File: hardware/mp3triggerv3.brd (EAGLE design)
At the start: 73.7 x 64.8 mm, 93 parts, among them J1 5.5x2.1mm Barrel, J10 M08X2, J3 USD-SOCKETNEW, J9 M10X2, U1 NCP1117, U2 MIC5323-3.3, U4 STM32F405RG, U5 PCM5100, U6 LM4990, Y1 8MHz

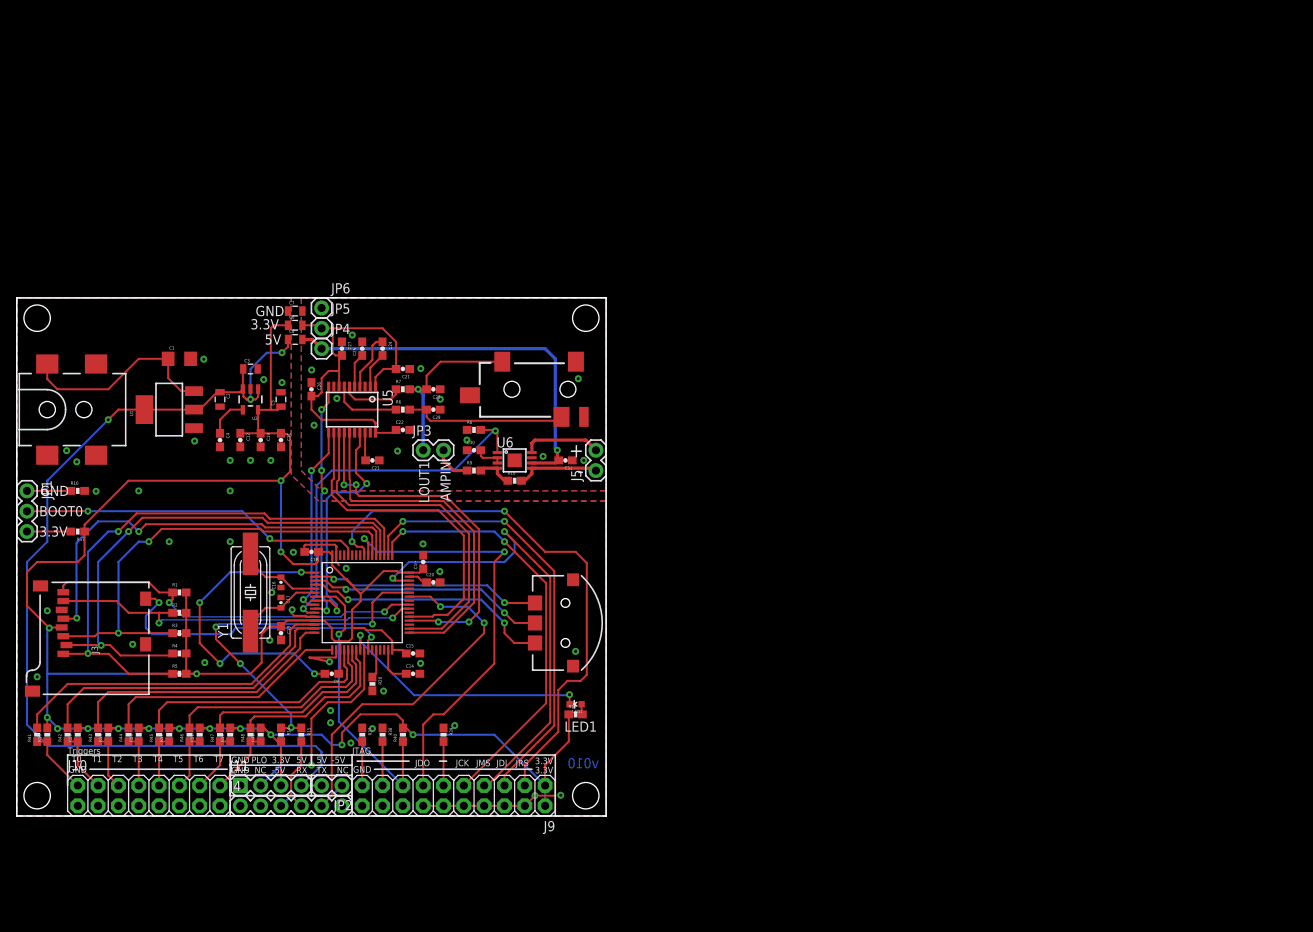
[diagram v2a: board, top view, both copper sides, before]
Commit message: v31, ready for review
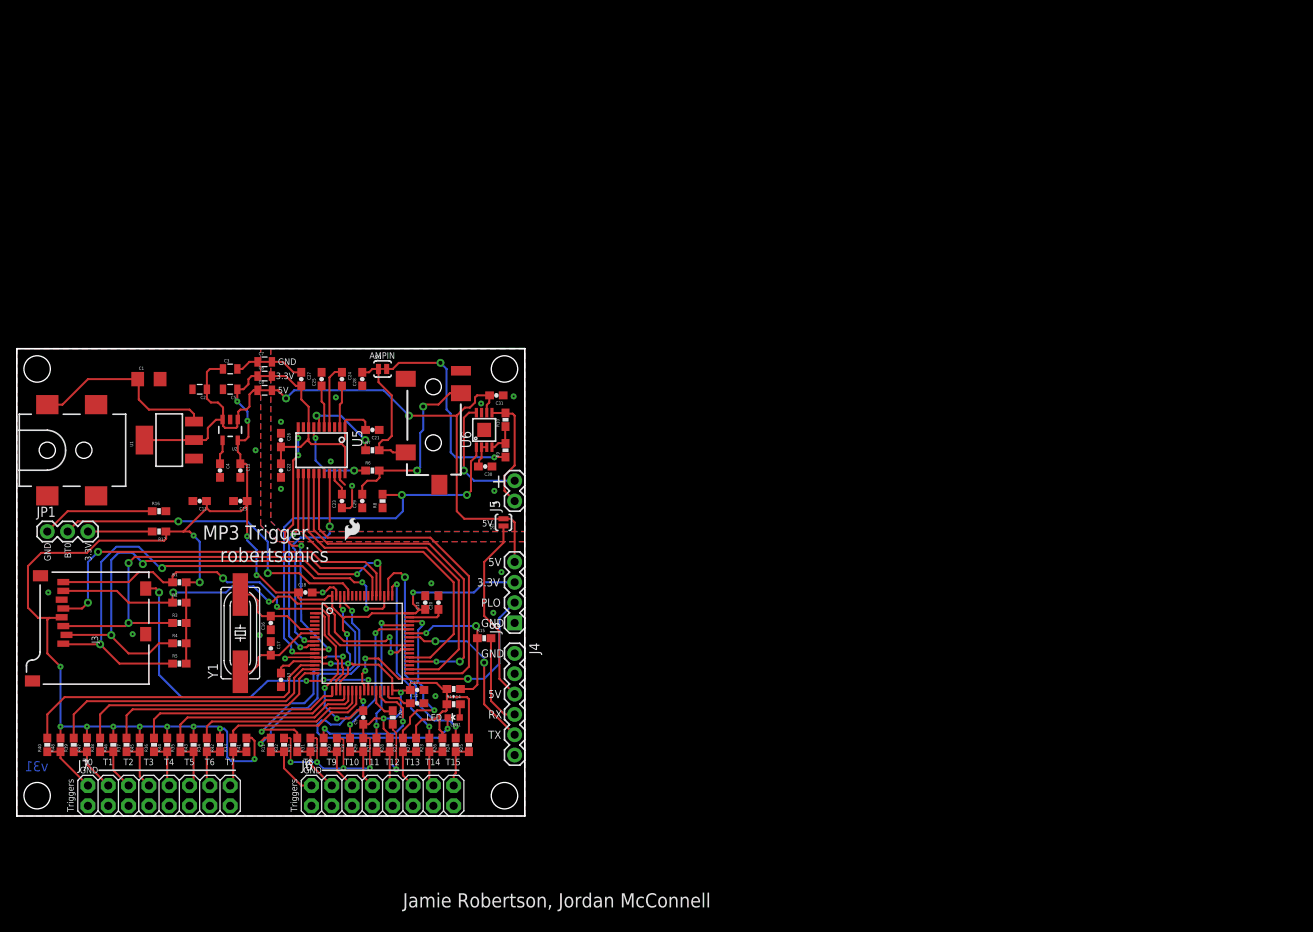
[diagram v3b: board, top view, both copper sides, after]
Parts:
- removed J10: M08X2, SparkFun-Connectors:2X8
- removed J11: (no value), SparkFun-Connectors:1X04
- removed J9: M10X2, SparkFun-Connectors:2X10
- removed JP2, JP3: (no value), SparkFun-Connectors:1X02
- removed JP4, JP5, JP6: M01PTH, SparkFun-Connectors:1X01
- removed R49, R50, R51, R52, R53, R54, R55, R56: 10K, SparkFun-Passives:0603-RES
- removed S1: NAV_SWITCHSMD, SparkFun-Electromechanical:NAV_SWITCH
- added CC_TEXT1: CREATIVE_COMMONS, SparkFun-Aesthetics:CREATIVE_COMMONS
- added J6, J7: M08X2, SparkFun-Connectors:2X8
- added J8: (no value), SparkFun-Connectors:1X04
- added LOGO1: OSHW-LOGOL, SparkFun-Aesthetics:OSHW-LOGO-L
- added LOGO2: LOGO-SFENEW, SparkFun-Aesthetics:SFE-NEW-WEBLOGO
- added LOGO3: LOGO-SFESK, SparkFun-Aesthetics:SFE-LOGO-FLAME
- added R11, R12, R13, R18, R21, R22, R23, R24, R33, R34, R35, R36: 100, SparkFun-Passives:0603-RES
- added R25, R26, R27, R28, R29, R30, R31, R32: 10K, SparkFun-Passives:0603-RES
- added SJ1: SOLDERJUMPERTRACE, SparkFun-Passives:SJ_2S-TRACE
- added SJ2: SOLDERJUMPERNO, SparkFun-Passives:SJ_2S-NO
- C16, C17: device SparkFun-Capacitors:0402-CAP -> SparkFun-Capacitors:0603-CAP
- R10: value 22K -> 10K
- R15, R37, R38, R39, R40: value 10K -> 100
- R41, R42, R43, R44, R45, R46, R47, R48: value 100 -> 10K
- moved R39 46.2 mm to (7.11, 8.89), turned to 90 degrees
- moved R40 44.5 mm to (3.81, 8.89)
- moved J4 39.2 mm to (62.2, 20.3), turned to 270 degrees
- moved R38 35.3 mm to (10.4, 8.89), turned to 90 degrees
- moved R37 29.5 mm to (13.7, 8.89), turned to 90 degrees
- moved R41 26.2 mm to (28.7, 8.89)
- moved R15 25.8 mm to (58.4, 22.2), turned to 0 degrees
- moved R48 23.8 mm to (5.46, 8.89)
- moved R14 22.3 mm to (54.6, 15.9), turned to 180 degrees
- moved J2 20.7 mm to (52.1, 57.1), turned to 270 degrees
- moved R42 19.1 mm to (25.4, 8.89)
- moved R47 16.7 mm to (8.76, 8.89)
- moved C22 16.1 mm to (33.0, 43.2), turned to 270 degrees
- moved LED1 15.3 mm to (54.6, 12.3)
- moved R19 15.3 mm to (54.6, 14.0)
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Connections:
- removed net JTCK: J9.9, U4.P$49
- removed net JTDI: J9.5, U4.P$50
- removed net JTDO: J9.13, U4.P$55
- removed net JTMS: J9.7, U4.P$46
- removed net JTRST: J9.3, U4.P$56
- removed net N$33: J9.17, R38.2
- removed net N$34: J9.11, R39.2
- removed net NAV1: S1.1, U4.P$2
- removed net NAV2: S1.2, U4.P$4
- removed net NAVT: S1.T, U4.P$3
- new net N$23: J6.4, R12.1, R31.1
- new net N$24: J6.6, R13.1, R30.1
- new net N$25: J6.8, R18.1, R29.1
- new net N$26: J6.10, R21.1, R28.1
- new net N$27: J6.12, R22.1, R27.1
- new net N$28: J6.14, R23.1, R26.1
- new net N$30: J6.16, R24.1, R25.1
- new net TRIG08: R11.2, U4.P$61
- new net TRIG09: R12.2, U4.P$62
- new net TRIG10: R13.2, U4.P$29
- new net TRIG11: R18.2, U4.P$44
- new net TRIG12: R21.2, U4.P$45
- new net TRIG13: R22.2, U4.P$46
- new net TRIG14: R23.2, U4.P$49
- new net TRIG15: R24.2, U4.P$50
- net +5V: now also J8.4, SJ2.2; no longer J11.4, JP2.2, JP4.1
- net AMPIN: now also SJ1.2; no longer JP3.2
- net GND: now also J6.1, J6.11, J6.13, J6.15, J6.3, J6.5, J6.7, J6.9, J7.1, J7.11, J7.13, J7.15, J7.3, J7.5, J7.7, J7.9, J8.1; no longer J10.1, J10.11, J10.13, J10.15, J10.3, J10.5, J10.7, J10.9, J11.1, J9.10, J9.12, J9.14, J9.16, J9.18, J9.20, J9.4, J9.6, J9.8, JP6.1, R37.1, R38.1, R39.1, S1.C
- net LOUTL: now also SJ1.1; no longer JP3.1
- net N$1: now also J6.2, R11.1, R32.1; no longer J9.19, R37.2
- net N$32: now also SJ2.1; no longer JP2.1
- net N$35: now also J7.2, R40.1, R48.1; no longer J10.2, R41.1, R56.1
- net N$36: now also J7.4, R39.1, R47.1; no longer J10.4, R42.1, R55.1
- net N$37: now also J7.6, R38.1, R46.1; no longer J10.6, R43.1, R54.1
- net N$38: now also J7.8, R37.1, R45.1; no longer J10.8, R44.1, R53.1
- net N$39: now also J7.10, R36.1, R44.1; no longer J10.10, R45.1, R52.1
- net N$40: now also J7.12, R35.1, R43.1; no longer J10.12, R46.1, R51.1
- net N$41: now also J7.14, R34.1, R42.1; no longer J10.14, R47.1, R50.1
- net N$42: now also J7.16, R33.1, R41.1; no longer J10.16, R48.1, R49.1
- net NRST: no longer J9.15, R40.1
- net PLAYOUT: now also J8.2; no longer J11.2
- net TRIG00: now also R40.2; no longer R41.2
- net TRIG01: now also R39.2; no longer R42.2
- net TRIG02: now also R38.2; no longer R43.2
- net TRIG03: now also R37.2; no longer R44.2
- net TRIG04: now also R36.2; no longer R45.2
- net TRIG05: now also R35.2; no longer R46.2
- net TRIG06: now also R34.2; no longer R47.2
- net TRIG07: now also R33.2; no longer R48.2
- net VCC: now also J8.3, R25.2, R26.2, R27.2, R28.2, R29.2, R30.2, R31.2, R32.2, R41.2, R42.2, R43.2, R44.2, R45.2, R46.2, R47.2, R48.2; no longer J11.3, J9.1, J9.2, JP5.1, R40.2, R49.2, R50.2, R51.2, R52.2, R53.2, R54.2, R55.2, R56.2
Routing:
- net +5V: track 173.0 -> 90.0 mm, vias 4 -> 2
- net JTRST: track 69.0 -> 0.00 mm, vias 2 -> 0
- net JTMS: track 59.6 -> 0.00 mm, vias 2 -> 0
- net JTDI: track 55.9 -> 0.00 mm, vias 2 -> 0
- net JTDO: track 54.6 -> 0.00 mm, vias 2 -> 0
- net JTCK: track 53.6 -> 0.00 mm, vias 2 -> 0
- net NRST: track 35.9 -> 0.00 mm, vias 1 -> 0
- net TRIG09: track 0.00 -> 31.7 mm, vias 0 -> 2
- net VCC: track 349.2 -> 317.6 mm, vias 15 -> 25
- net NAV2: track 31.3 -> 0.00 mm, vias 2 -> 0
- net NAVT: track 29.7 -> 0.00 mm, vias 2 -> 0
- net TRIG08: track 0.00 -> 29.6 mm, vias 0 -> 2
- net RXD: track 47.8 -> 18.5 mm, vias 4 -> 2
- net NAV1: track 28.9 -> 0.00 mm, vias 2 -> 0
- net TRIG15: track 0.00 -> 28.6 mm, vias 0 -> 2
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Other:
- board size 73.7 x 64.8 mm -> 63.5 x 58.4 mm
- board text added: "BT0"
- board text added: "Jamie Robertson, Jordan McConnell"
- board text added: "LED"
- board text added: "MP3 Trigger"
- board text added: "T10"
- board text added: "T11"
- board text added: "T12"
- board text added: "T13"
- board text added: "T14"
- board text added: "T15"
- board text added: "T8"
- board text added: "T9"
- board text added: "robertsonics"
- board text added: "v31"
- board text removed: "-5V"
- board text removed: "BOOT0"
- board text removed: "JCK"
- board text removed: "JDI"
- board text removed: "JDO"
- board text removed: "JMS"
- board text removed: "JRS"
- board text removed: "JTAG"
- board text removed: "LED1"
- board text removed: "LOUT1"
- board text removed: "NC"
- board text removed: "v010"
